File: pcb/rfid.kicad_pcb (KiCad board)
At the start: 2 copper layers, 26.2 x 64.5 mm, 55 parts, among them IC1 EM4095, IC2 ATTINY13A-SS, J1 USB

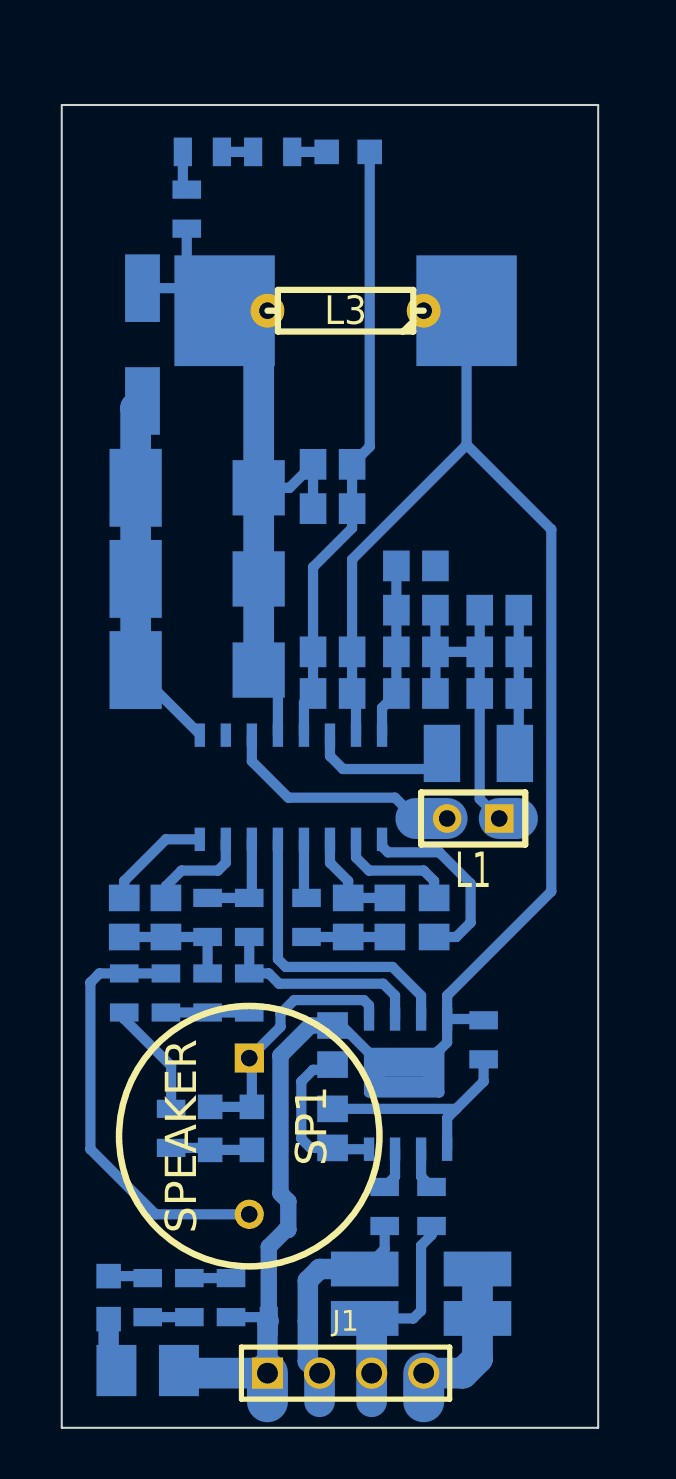
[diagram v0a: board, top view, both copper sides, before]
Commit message: finalising pcb routing
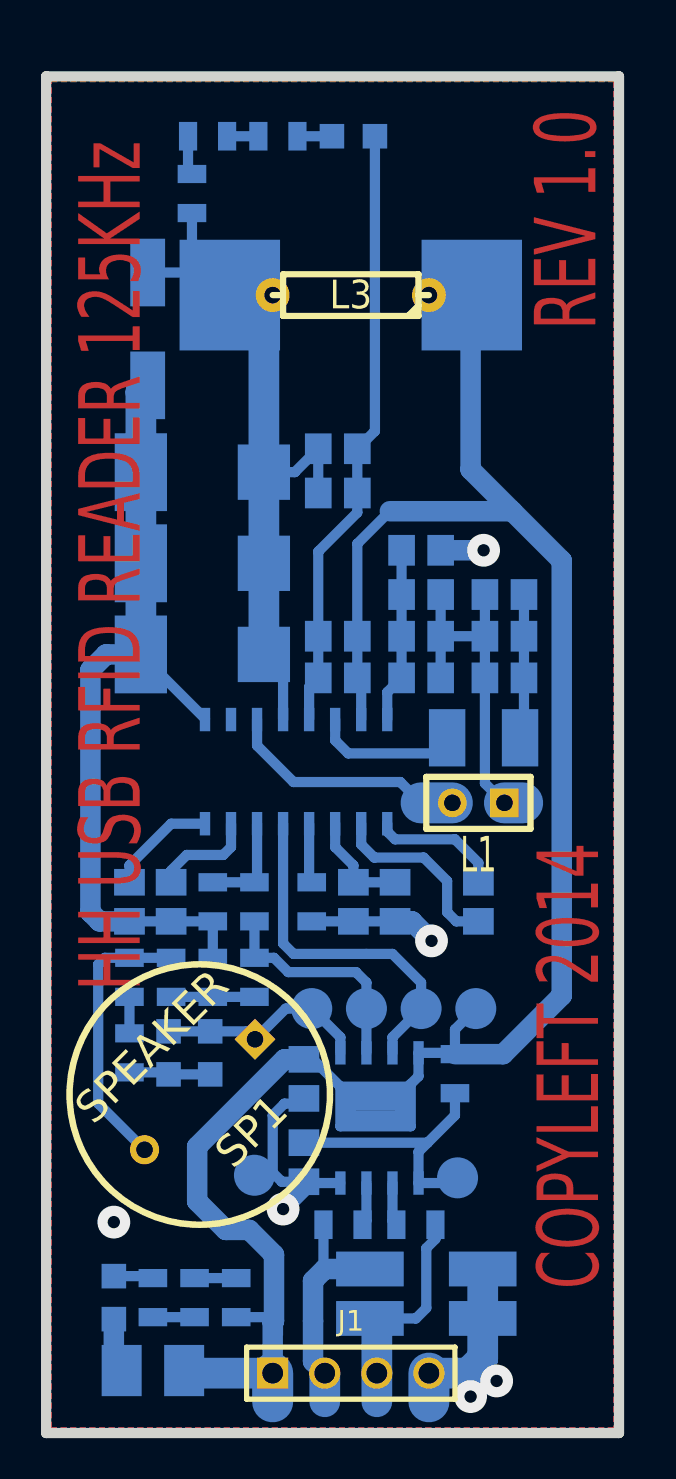
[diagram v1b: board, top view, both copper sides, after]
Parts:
- added P1: CONN_1, smd_pad_2mm, B.Cu at (217.7, 166.6)
- added P2: CONN_1, smd_pad_2mm, B.Cu at (207.8, 166.5)
- added P3: CONN_1, smd_pad_2mm, B.Cu at (215.9, 158.4)
- added P4: CONN_1, smd_pad_2mm, B.Cu at (210.6, 158.4)
- added P5: CONN_1, smd_pad_2mm, B.Cu at (213.2, 158.4)
- added P6: CONN_1, smd_pad_2mm, B.Cu at (218.6, 158.4)
- moved D3 4.21 mm to (203.6, 160.5)
- moved D4 4.21 mm to (205.6, 160.5)
- moved R13 4.21 mm to (201.7, 160.5)
- moved SP1 3.15 mm to (205.1, 162.6), turned to 225 degrees
- moved C8 2.29 mm to (218.7, 153.2), turned to 90 degrees
- moved R4 2.22 mm to (212.1, 168.9), turned to 180 degrees
- moved R10 2.16 mm to (217.6, 161.5)
- moved C15 2.16 mm to (210.2, 161.8)
- moved IC2 2.16 mm to (213.9, 163.7)
- moved C13 2.16 mm to (210.2, 165.9)
- moved R3 1.17 mm to (215.6, 168.9), turned to 0 degrees
- moved C11 0.80 mm to (212.6, 153.2)
- moved C16 0.80 mm to (211.8, 142.2)
- moved C2 0.80 mm to (215.9, 142.2)
- moved C20 0.80 mm to (211.8, 133.2)
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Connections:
- net N-000005 renamed /RST
- D3 pad 2: N-0000025 (its old number) -> /MOSI
- D4 pad 1: N-0000025 (its old number) -> /MOSI
- IC1 pad 13: N-0000012 (its old number) -> /SCK
- IC2 pad 5: N-0000025 (its old number) -> /MOSI
- IC2 pad 6: N-0000019 (its old number) -> /MISO
- IC2 pad 7: N-0000012 (its old number) -> /SCK
- R7 pad 1: N-0000019 (its old number) -> /MISO
- R8 pad 2: N-0000019 (its old number) -> /MISO
- SP1 pad 1: N-0000025 (its old number) -> /MOSI
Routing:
- net GND: track 76.8 -> 102.1 mm, vias 0 -> 5
- net /SCK: track 0.00 -> 17.4 mm
- net N-0000012 (its old number): track 14.7 -> 0.00 mm
- net N-0000025 (its old number): track 12.6 -> 0.00 mm
- net /MISO: track 0.00 -> 11.2 mm
- net /MOSI: track 0.00 -> 10.5 mm
- net N-0000019 (its old number): track 10.5 -> 0.00 mm
- net +5V: track 118.1 -> 126.1 mm
- net N-0000017: track 21.1 -> 13.7 mm
- net N-0000019: track 5.71 -> 1.84 mm
- net N-0000024: track 6.00 -> 9.18 mm
- net N-0000014: track 9.39 -> 6.41 mm
- net /RST: track 10.9 -> 12.9 mm
- net (no net): vias 0 -> 1
- added copper zone on B.Cu, net GND
- added copper zone on F.Cu, net GND
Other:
- board size 26.2 x 64.5 mm -> 27.9 x 66.2 mm
- board text added: "COPYLEFT 2014"
- board text added: "HH USB RFID READER 125KHz"
- board text added: "REV 1.0"
